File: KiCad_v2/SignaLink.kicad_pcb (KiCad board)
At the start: 2 copper layers, 56.5 x 42.3 mm, 66 parts, among them Q1 MMBT3904, SW1 SW_Wake, U1 DM-OLED096-636, U2 ESP32-C3_SUPERMINI_TH, U3 MIC94063YC6-TR, U4 CM4102008, U5 LT8582EDKD-PBF, U6 MCP73871, U7 LM3940IMP-3.3, U8 BNO085, U9 MPU-6050

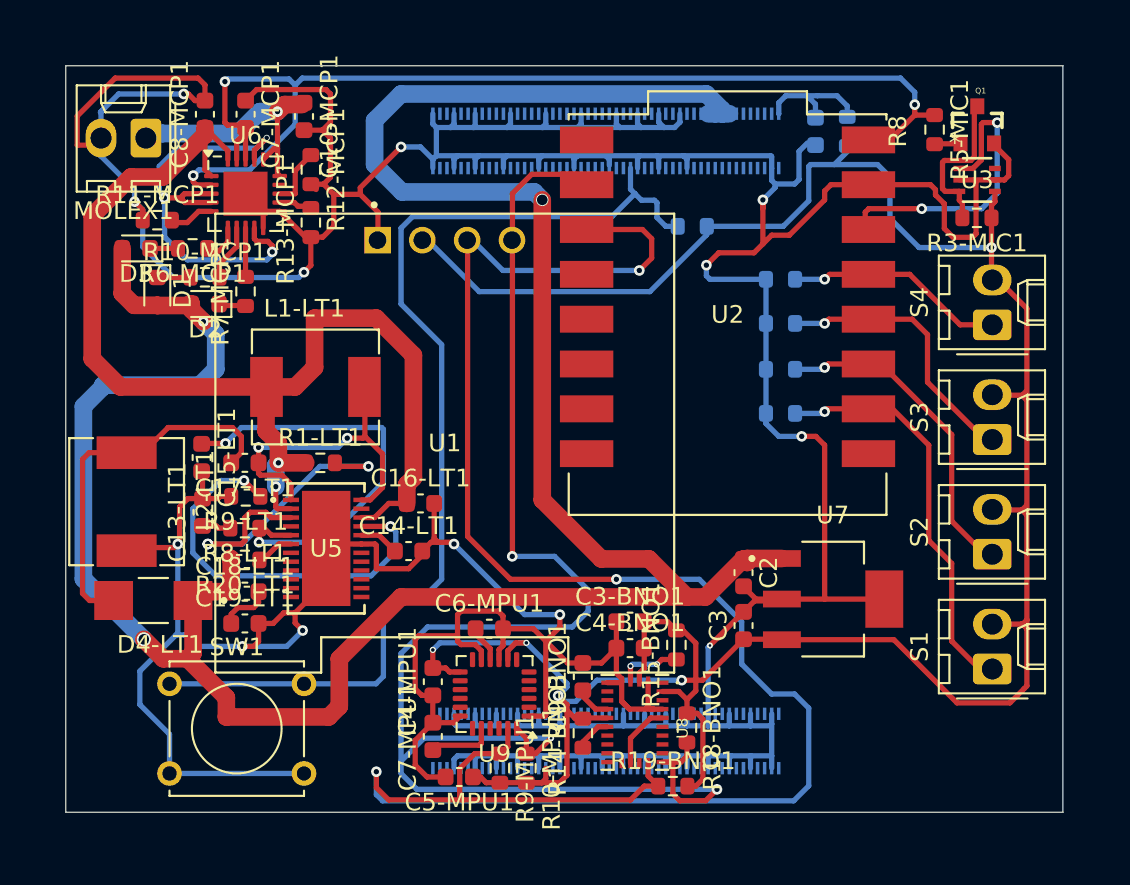
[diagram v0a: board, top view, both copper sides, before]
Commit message: feat: subo version final del pcb y sumo logos
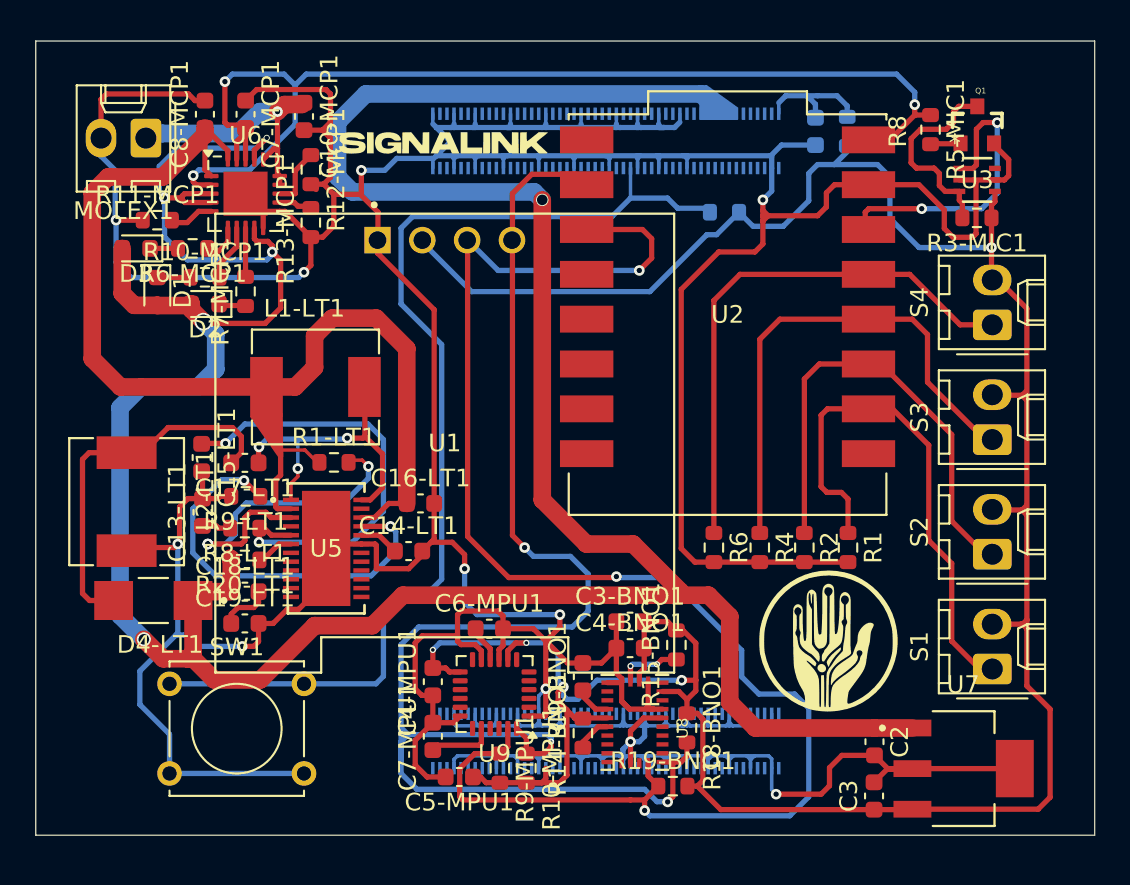
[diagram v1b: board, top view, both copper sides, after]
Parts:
- added G***: LOGO, Custom_Footprints:signaa, F.Cu at (63.7, 81.5)
- added G***: LOGO, Custom_Footprints:signaaaaaaaaaaaa, F.Cu at (41.9, 53.7)
- R1, R2, R4, R6: moved to F.Cu
- moved R6 15.7 mm to (57.2, 76.2), turned to -90 degrees
- moved R4 12.8 mm to (59.8, 76.2), turned to -90 degrees
- moved C3 12.2 mm to (66.3, 90.3)
- moved U7 12.1 mm to (71.4, 88.7)
- moved C2 12.1 mm to (66.3, 87.2)
- moved R2 10.2 mm to (62.4, 76.2), turned to -90 degrees
- moved R1 8.51 mm to (64.8, 76.2), turned to -90 degrees
- moved R7 1.99 mm to (57.8, 57.2)
- moved R1-LT1 0.78 mm to (35.7, 71.4)
- moved R5-MIC1 0.23 mm to (69.5, 52.5)
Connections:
- U6 pad 17: /5V -> +5V
- U6 pad 3: /5V -> +5V
- U6 pad 4: /5V -> +5V
- U6 pad 9: /5V -> +5V
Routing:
- net +5V: track 148.4 -> 189.7 mm, vias 3 -> 6
- net /5V: track 26.1 -> 0.00 mm, vias 3 -> 0
- net /SCL: track 114.2 -> 92.6 mm
- net GND: track 388.9 -> 408.1 mm, vias 13 -> 11
- net /A4: track 13.0 -> 31.2 mm, vias 1 -> 0
- net /A3: track 16.3 -> 29.6 mm, vias 1 -> 0
- net /A2: track 19.1 -> 27.5 mm, vias 1 -> 0
- net +3.3V: track 156.4 -> 163.7 mm
- net /A1: track 24.0 -> 30.4 mm, vias 1 -> 0
- net Net-(U3-EN): track 8.96 -> 12.0 mm
- net /SDA: track 87.9 -> 85.4 mm
- net /power_supply/OUT_MCP: track 66.0 -> 67.2 mm, vias 2 -> 0
- net Net-(U4A-GPIO2): track 60.1 -> 61.0 mm
- net Net-(U5-VC1): track 25.1 -> 25.9 mm
- net Net-(MOLEX1-Pin_1): track 15.5 -> 16.0 mm
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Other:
- board size 56.5 x 42.3 mm -> 60 x 45 mm
